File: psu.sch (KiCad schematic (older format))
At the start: 18 parts, among them U7 LM2596S-3.3, U9 LM7805

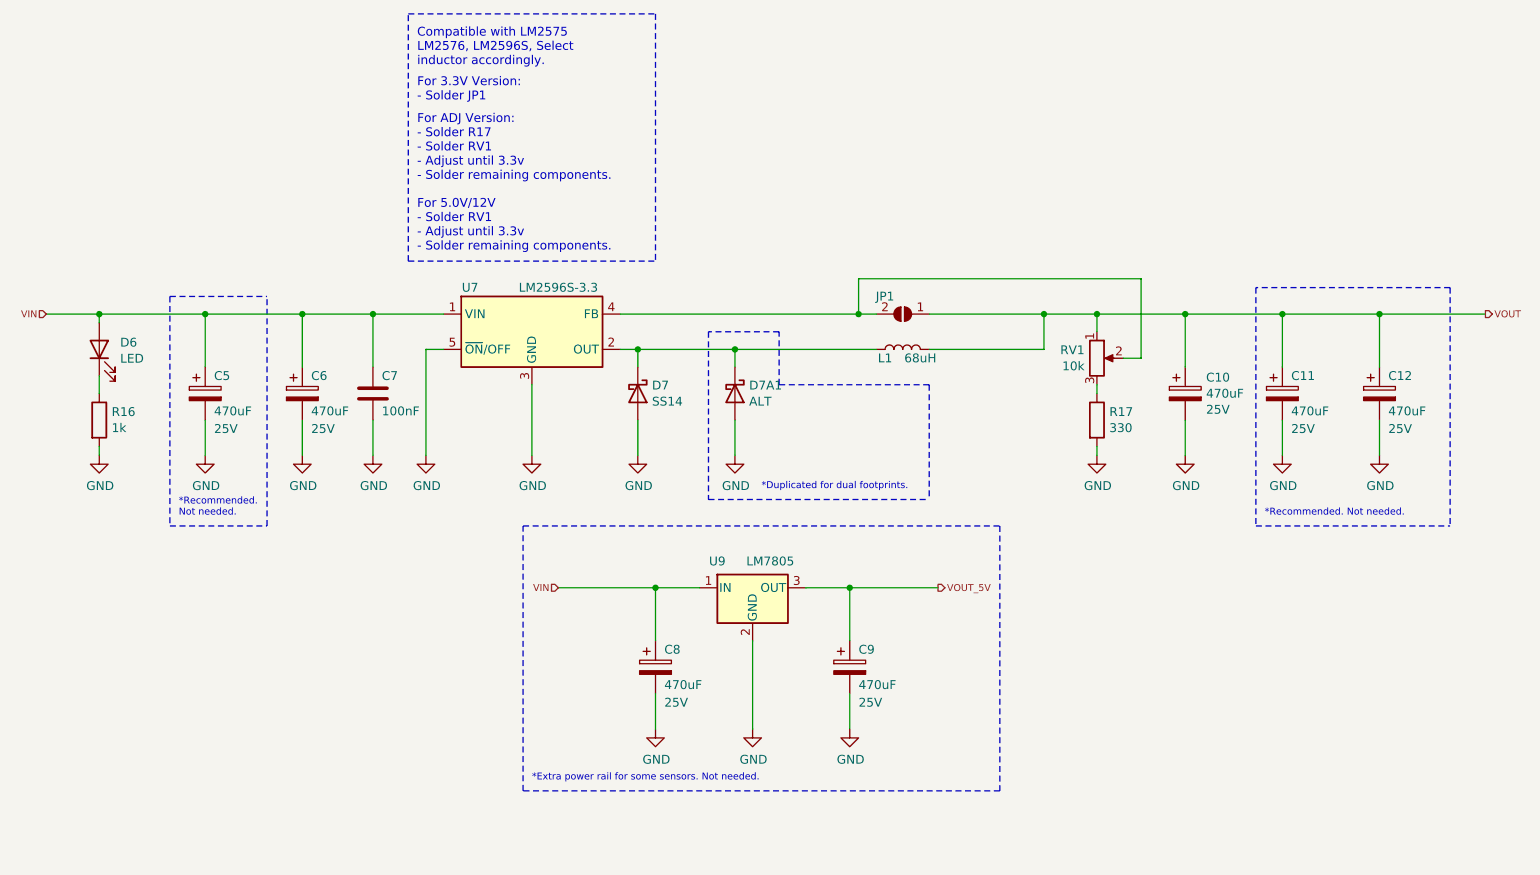
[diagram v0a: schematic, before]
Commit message: Several changes
Usando stock de http://tienda.ityt.com.ar/
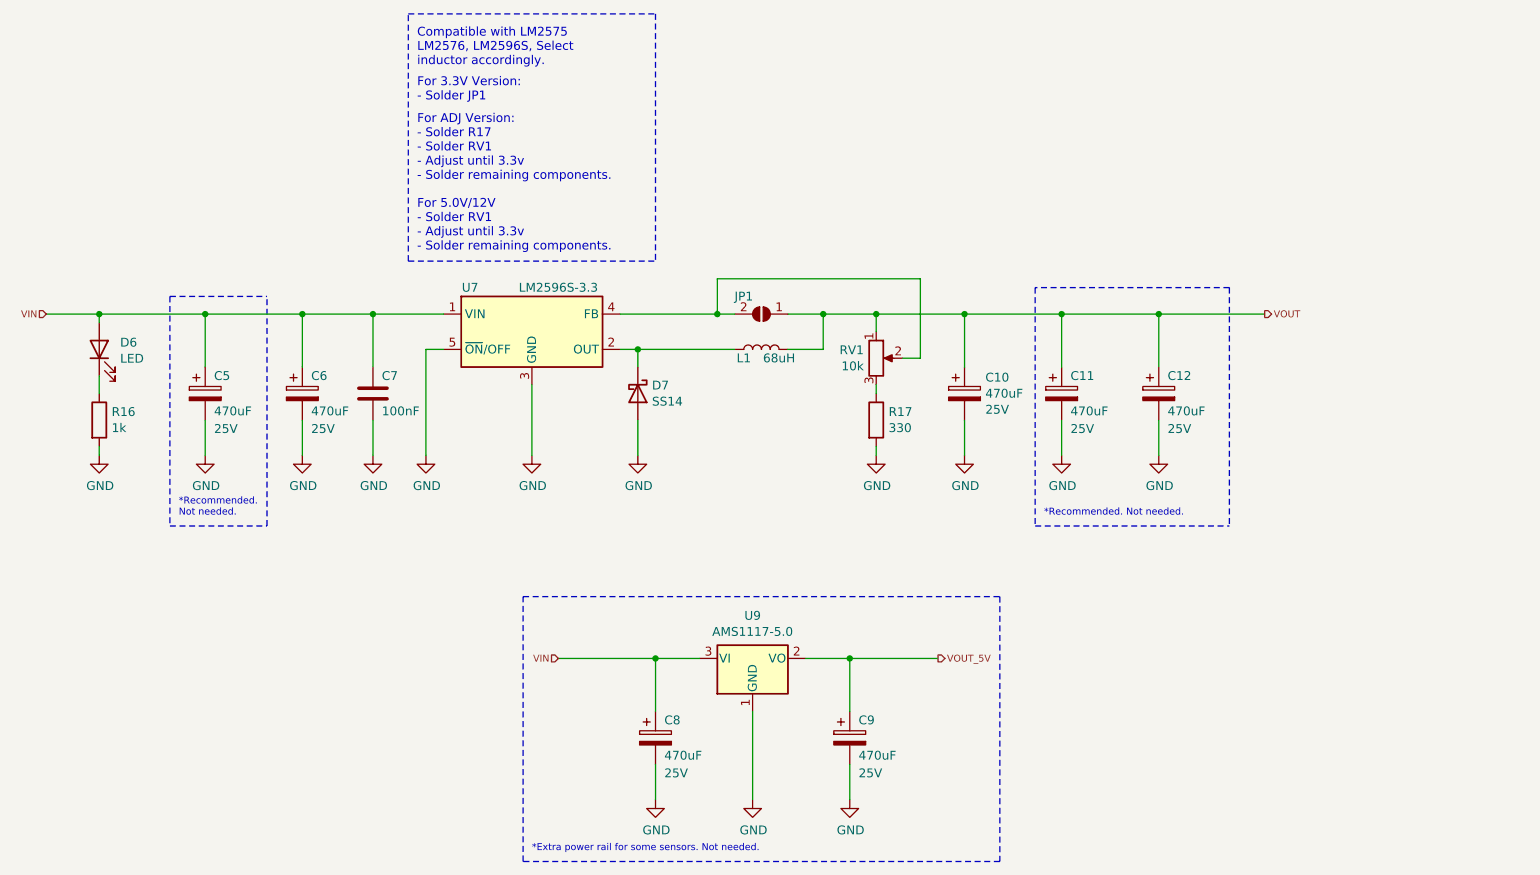
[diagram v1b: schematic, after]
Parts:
- removed D7A1: ALT, Diode_THT:D_DO-201_P12.70mm_Horizontal, symbol Diode:1N5822
- removed U9: LM7805, Package_TO_SOT_THT:TO-220-3_Vertical, symbol Regulator_Linear:L7805
- added U9: AMS1117-5.0, Package_TO_SOT_SMD:SOT-223-3_TabPin2, symbol Regulator_Linear:AMS1117-5.0
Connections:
- net GND: now also U9.1 (GND)
- net VIN: now also U9.3 (VI)
- net VOUT_5V: now also U9.2 (VO)
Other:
- note removed: "*Duplicated for dual footprints."
- moved on the sheet: C10, C11, C12, C8, C9, JP1, L1, R17, RV1
